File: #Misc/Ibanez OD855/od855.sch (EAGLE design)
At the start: 77 parts, among them IC101 RC4558, Q101 2SC1815BL, Q102 1SK44SP, Q103 2SC1815BL, Q104 2SK44SP, Q105 2SC1815BL, Q106 2SC1815BL, Q107 2SC1815BL, SW1 MOMENTARY

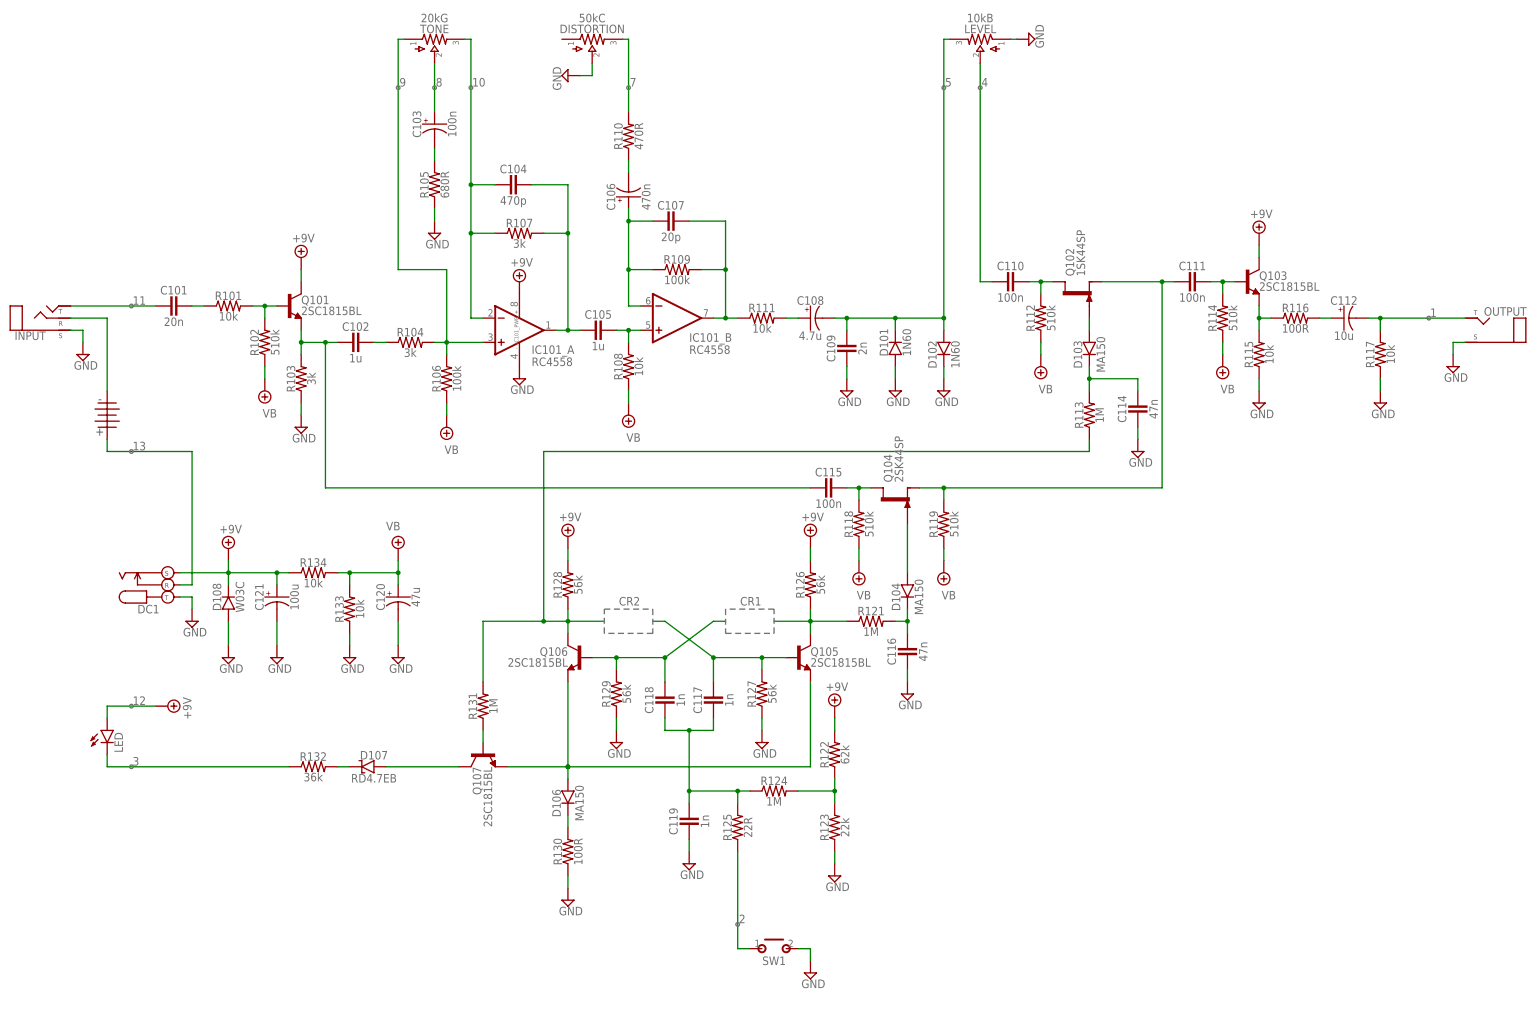
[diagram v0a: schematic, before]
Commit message: 20180125
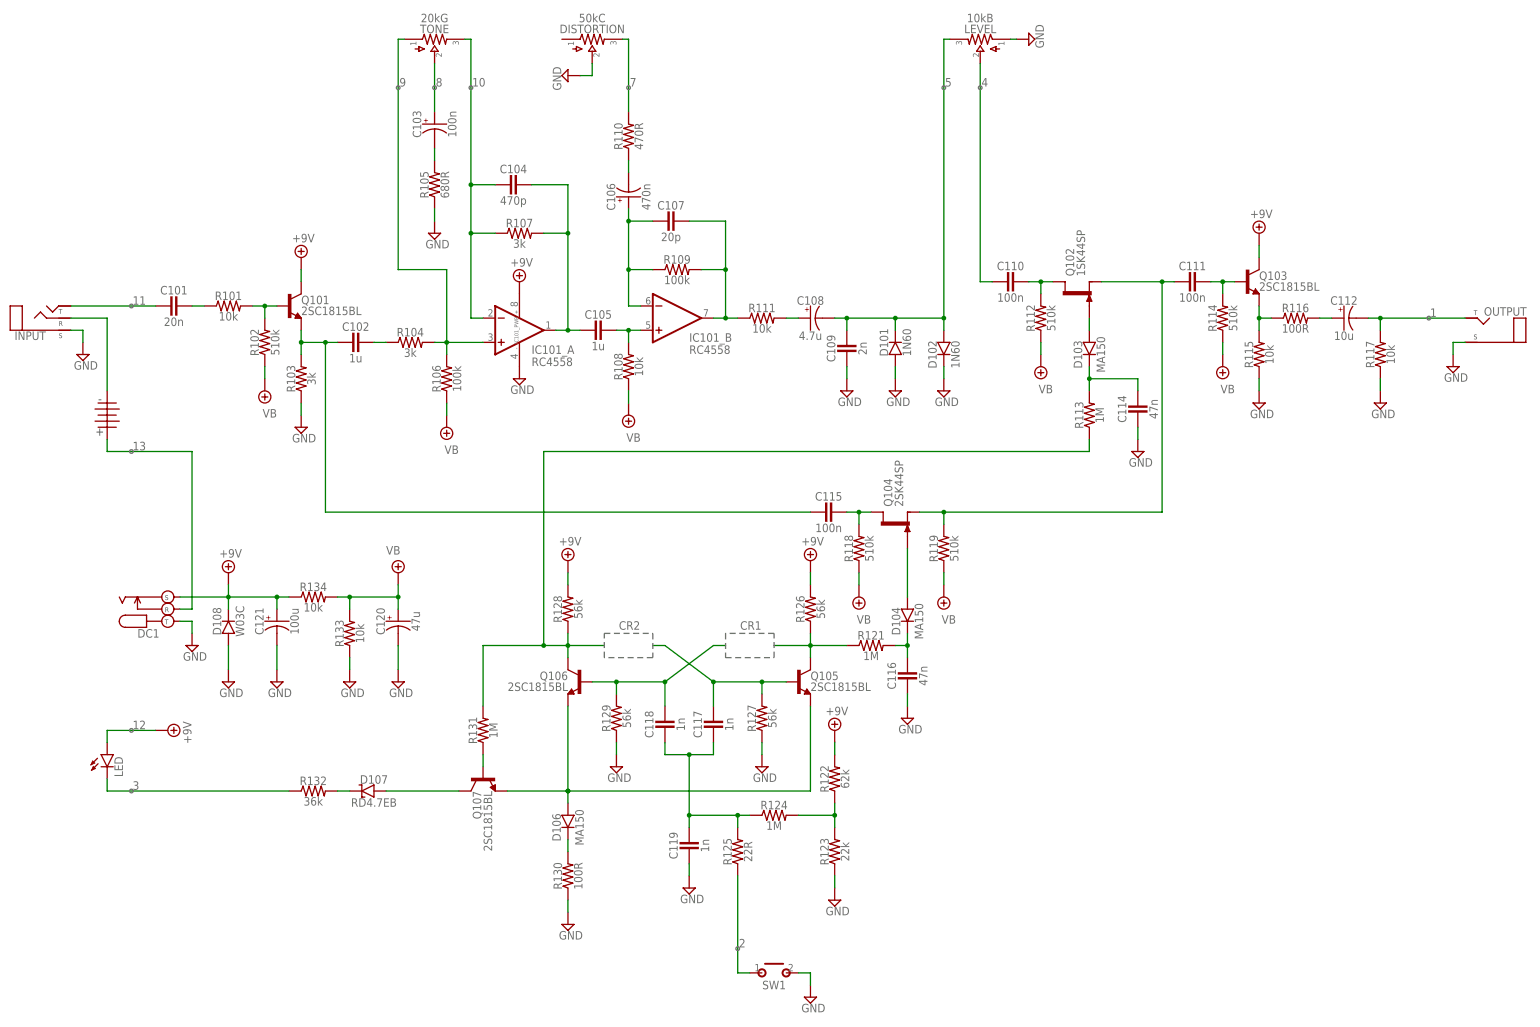
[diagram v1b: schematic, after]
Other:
- moved on the sheet: C115, C116, C117, C118, C119, C120, C121, D104, D106, D107, D108, DC1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
